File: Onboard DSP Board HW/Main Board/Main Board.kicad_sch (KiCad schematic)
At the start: 92 parts, among them J1 Bridge Pickup, J2 Neck Pickup, J3 Battery, J4 Output Jack, J5 Debug Connector, U1 TPS7A2033PDBVR, U2 TPS63020DSJR, U3 XLV320ADC5140IRTWR, U4 XLV320ADC5140IRTWR, U5 E104-BT5032A, U6 PCM5102, U8 TP4054

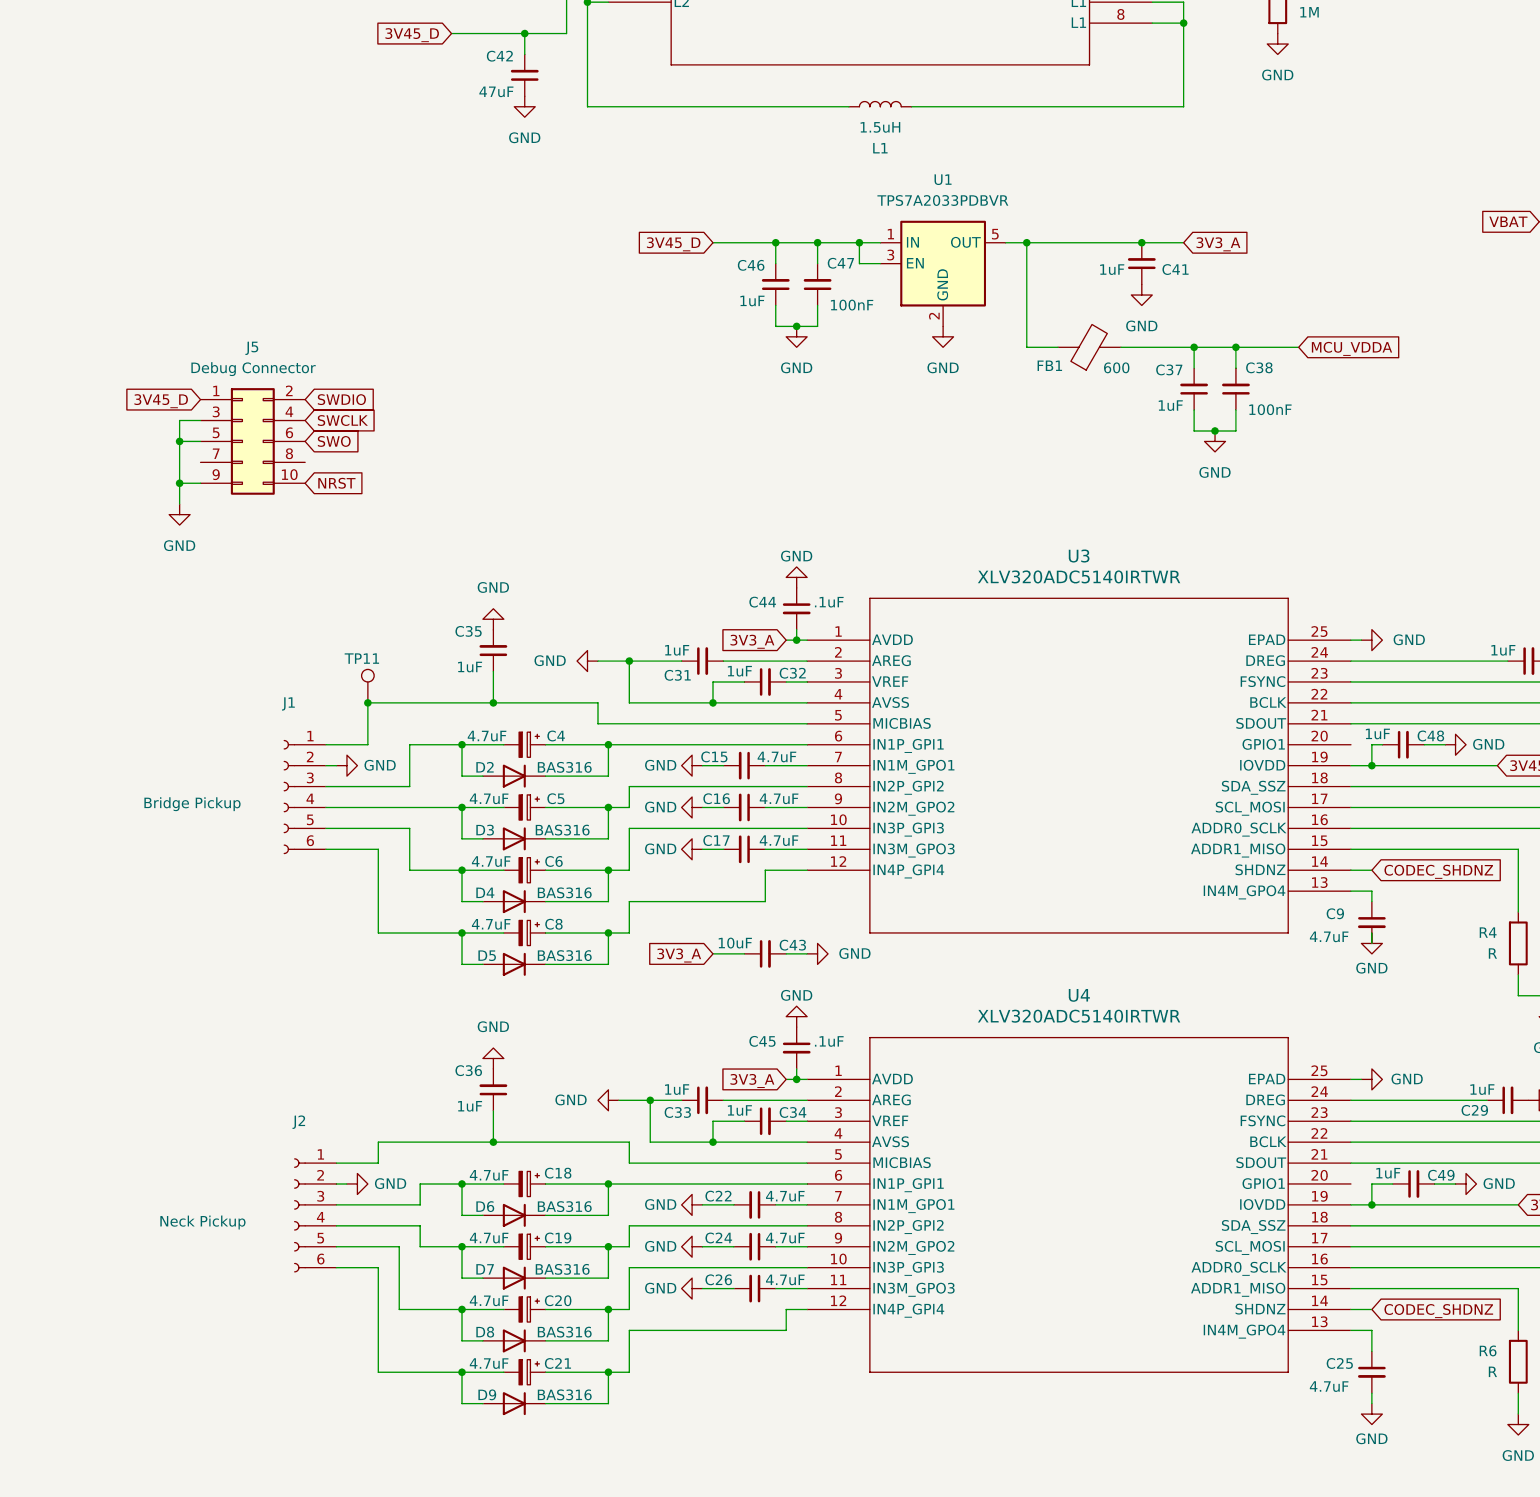
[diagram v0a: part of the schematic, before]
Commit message: WIP on DSP, add connectors
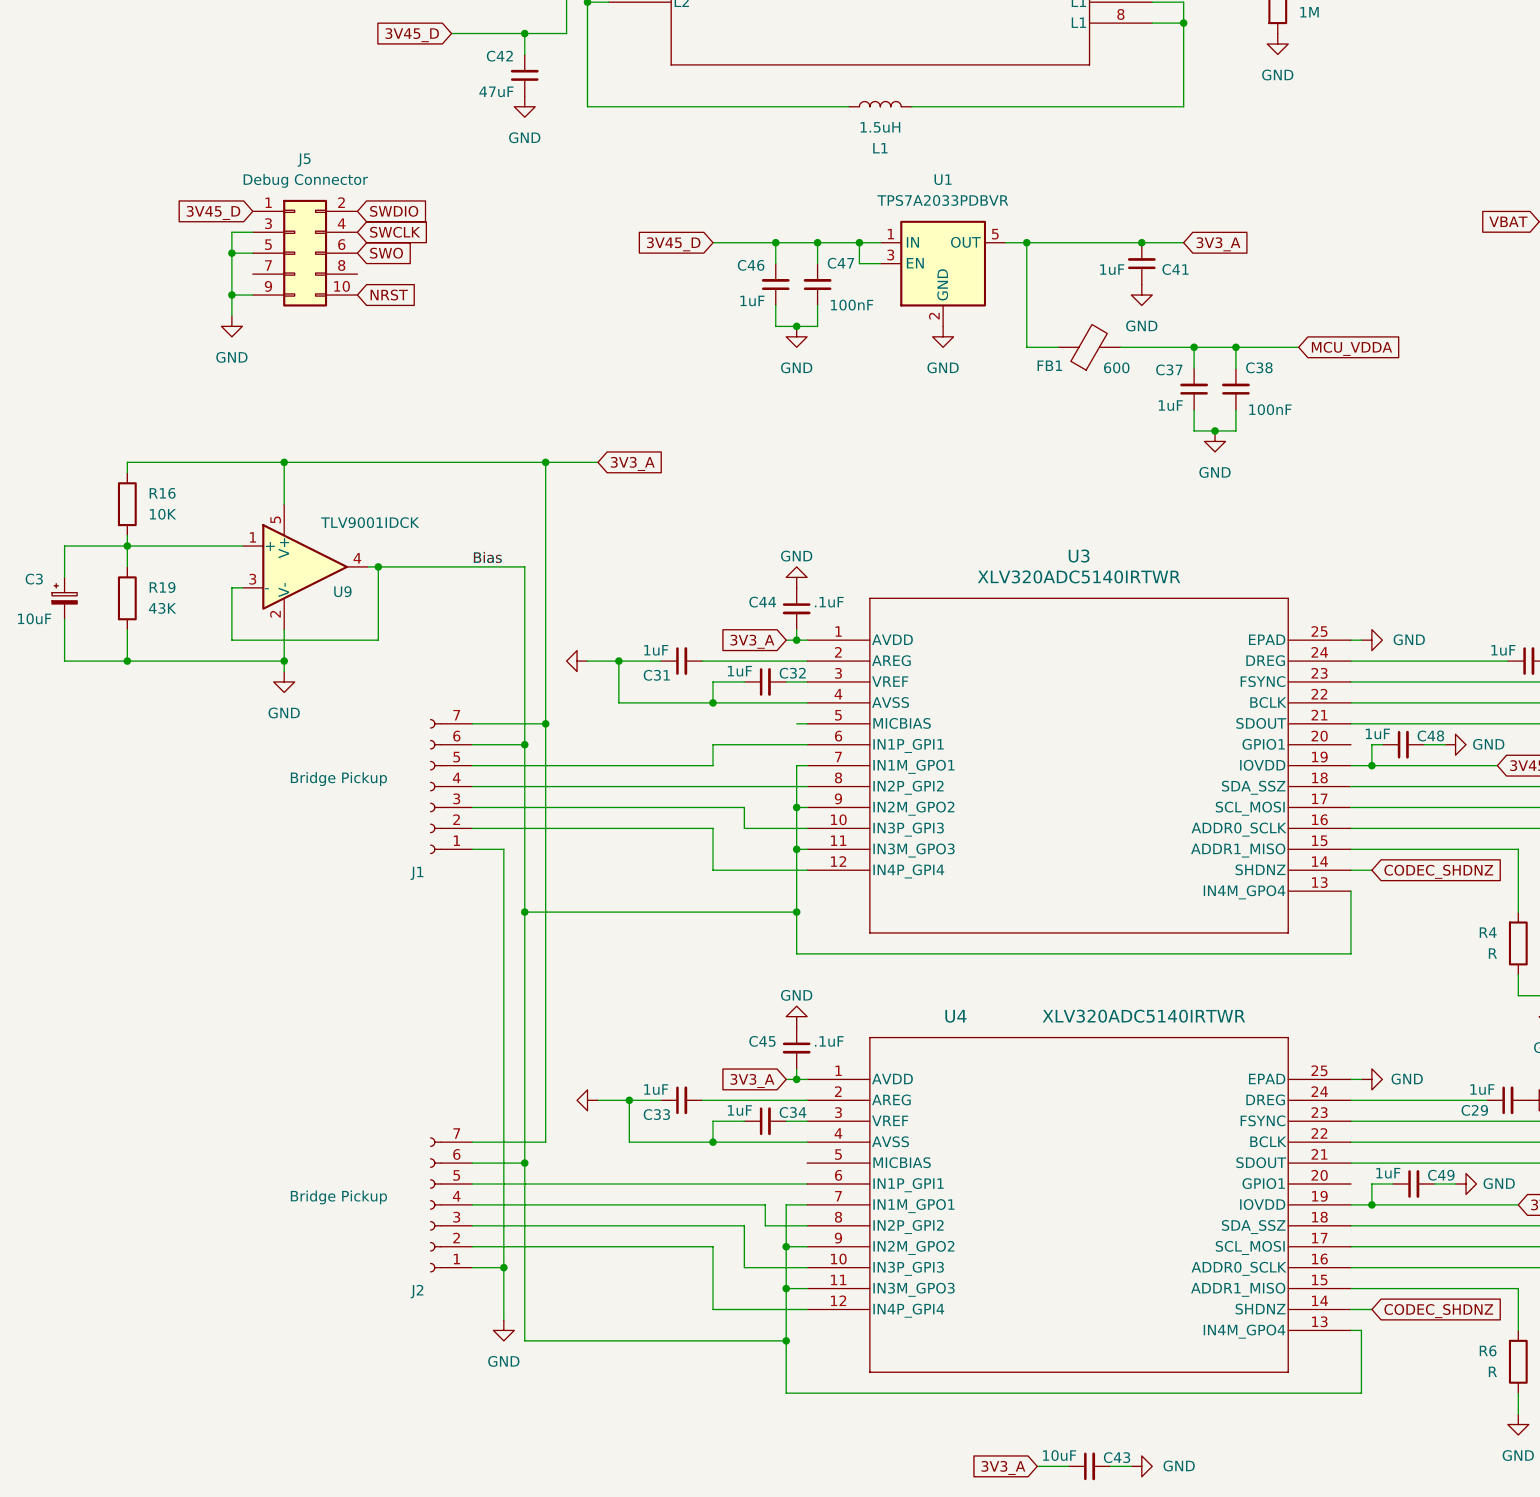
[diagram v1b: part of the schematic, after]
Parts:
- removed C15, C16, C17, C22, C24, C25, C26, C9: 4.7uF, Capacitor_SMD:C_0402_1005Metric, symbol Device:C_Small
- removed C18, C19, C20, C21, C4, C5, C6, C8: 4.7uF, Capacitor_SMD:C_1206_3216Metric, symbol Device:C_Polarized_Small
- removed C35, C36: 1uF, Capacitor_SMD:C_0402_1005Metric, symbol Device:C_Small
- removed D2, D3, D4, D5, D6, D7, D8, D9: BAS316, Diode_SMD:D_SOD-323, symbol Diode:1N914
- removed J1: Bridge Pickup, Connector_PinHeader_2.54mm:PinHeader_1x06_P2.54mm_Vertical, symbol Connector:Conn_01x06_Socket
- removed J2: Neck Pickup, Connector_PinHeader_2.54mm:PinHeader_1x06_P2.54mm_Vertical, symbol Connector:Conn_01x06_Socket
- removed TP11: (no value), symbol Connector:TestPoint
- added C3: 10uF, Capacitor_SMD:C_1206_3216Metric, symbol Device:C_Polarized_Small
- added J1, J2: Bridge Pickup, Connector_PinHeader_2.00mm:PinHeader_1x07_P2.00mm_Horizontal, symbol Connector:Conn_01x07_Socket
- added R16: 10K, Resistor_SMD:R_0402_1005Metric, symbol Device:R
- added R19: 43K, Resistor_SMD:R_0402_1005Metric, symbol Device:R
- added U9: TLV9001IDCK, Package_TO_SOT_SMD:SOT-353_SC-70-5, symbol Amplifier_Operational:TLV9001IDCK
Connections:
- net 3V3_A: now also J1.7 (Pin_7), J2.7 (Pin_7), R16.1, U9.5 (V+)
- net GND: now also C3.2, J1.1 (Pin_1), J2.1 (Pin_1), R19.2, U9.2 (V-)
- net at U4.10 (IN3P_GPI3): now also J2.3 (Pin_3)
- net at U3.8 (IN2P_GPI2): now also J1.4 (Pin_4)
- net at U3.6 (IN1P_GPI1): now also J1.5 (Pin_5)
- net at U4.6 (IN1P_GPI1): now also J2.5 (Pin_5)
- net Bias: now reaches U3.7 (IN1M_GPO1)
- net Bias: now also U3.11 (IN3M_GPO3), U3.13 (IN4M_GPO4), U3.9 (IN2M_GPO2), U4.11 (IN3M_GPO3), U4.13 (IN4M_GPO4), U4.7 (IN1M_GPO1), U4.9 (IN2M_GPO2), J1.6 (Pin_6), J2.6 (Pin_6), U9.3 (-), U9.4
- net at U3.10 (IN3P_GPI3): now also J1.3 (Pin_3)
- net at U4.12 (IN4P_GPI4): now also J2.2 (Pin_2)
- net at U3.12 (IN4P_GPI4): now also J1.2 (Pin_2)
- net at U4.8 (IN2P_GPI2): now also J2.4 (Pin_4)
- new net: C3.1, R16.2, R19.1, U9.1 (+)
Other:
- moved on the sheet: C31, C43, J5

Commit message: WIP
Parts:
- TP12, TP13, TP14: footprint (none) -> AWV:TestPoint_Plated_Hole_ID4_OD7.0mm
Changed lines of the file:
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@@
 			)
 		)
-		(property "Footprint" ""
+		(property "Footprint" "AWV:TestPoint_Plated_Hole_ID4_OD7.0mm"
 			(at 257.81 133.35 0)
 			(hide yes)
@@
 			)
 		)
-		(property "Footprint" ""
+		(property "Footprint" "AWV:TestPoint_Plated_Hole_ID4_OD7.0mm"
 			(at 270.51 133.35 0)
 			(hide yes)
@@
 			)
 		)
-		(property "Footprint" ""
+		(property "Footprint" "AWV:TestPoint_Plated_Hole_ID4_OD7.0mm"
 			(at 264.16 133.35 0)
 			(hide yes)
